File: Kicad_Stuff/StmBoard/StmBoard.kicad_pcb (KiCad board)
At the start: 4 copper layers, 103.6 x 50.6 mm, 46 parts, among them J1 USB_B_Mini, SW1 SW_DIP_x01, SW2 SW_DIP_x01, SW3 SW_DIP_x01, SW4 SW_DIP_x01, SW5 SW_DIP_x01, SW6 SW_DIP_x01, SW7 SW_DIP_x01, SW8 SW_DIP_x01, SW9 SW_DIP_x01, U1 STM32G031K8Tx, U13 MCP2221AxST, U2 LIS3DH, U8 MIC5504-3.3YM5, U9 L78L05_SO8, Y1 32Khz LSE

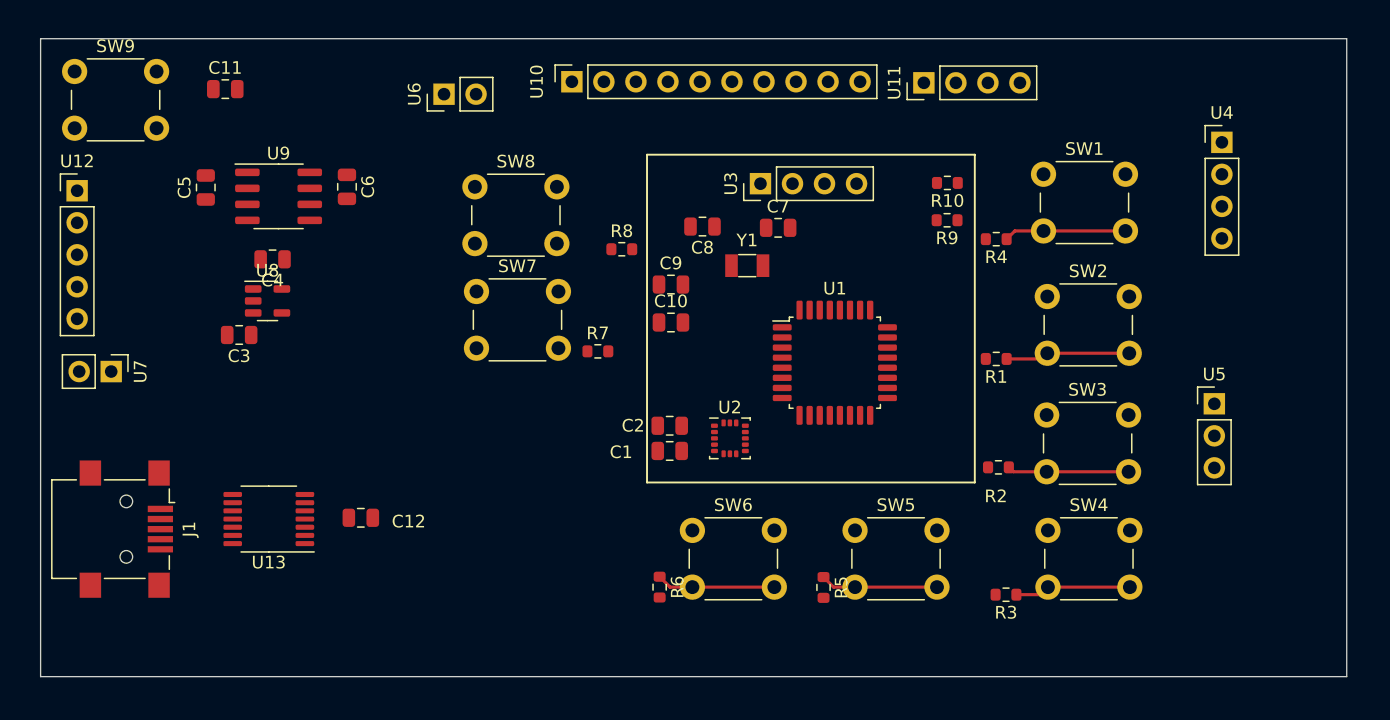
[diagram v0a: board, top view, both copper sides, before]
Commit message: quick commit
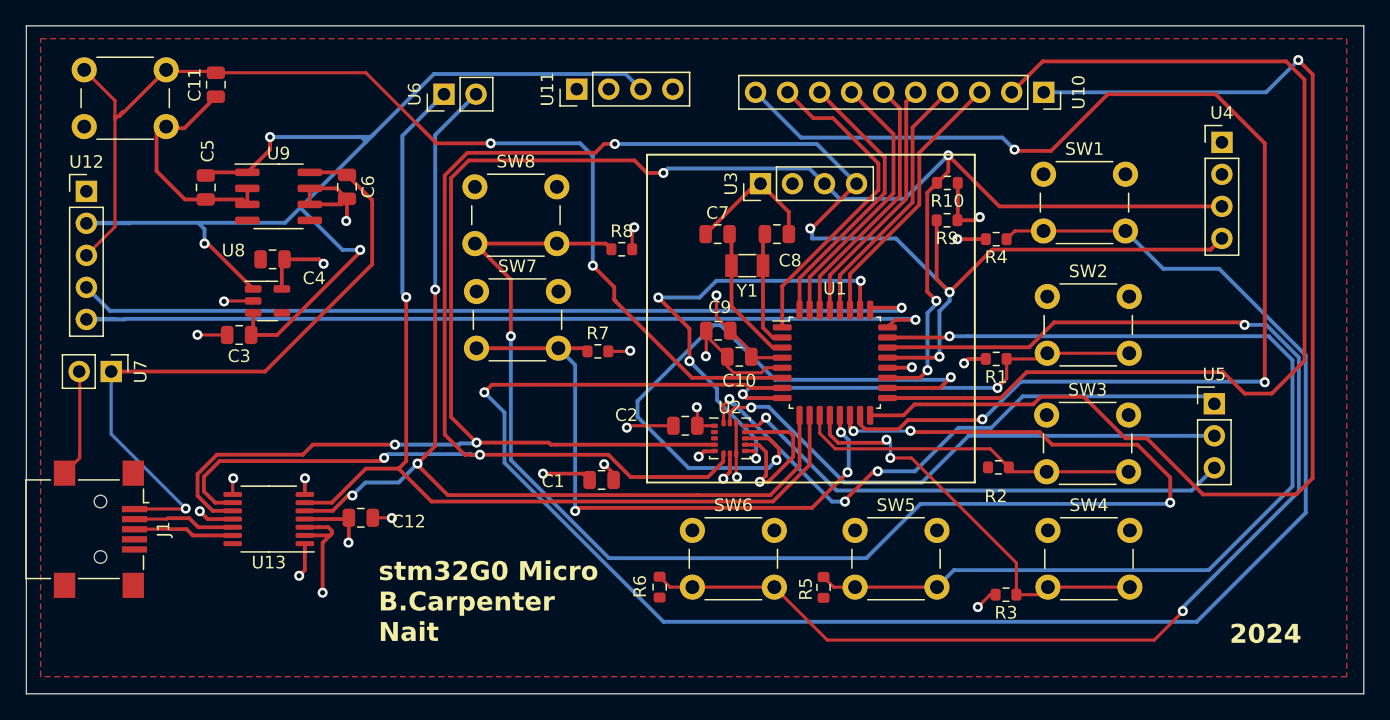
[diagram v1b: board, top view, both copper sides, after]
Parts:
- moved U10 37.4 mm to (154.3, 80.3), turned to -90 degrees
- moved U11 27.5 mm to (117.2, 80.1)
- moved C10 6.06 mm to (130.1, 101.3)
- moved C8 5.93 mm to (133.1, 91.6)
- moved C1 5.87 mm to (119.2, 111.1)
- moved C9 5.24 mm to (128.4, 99.3)
- moved C7 4.83 mm to (128.4, 91.6)
- moved J1 2.05 mm to (79.5, 115.0)
- moved C2 1.24 mm to (125.8, 106.8)
- moved C11 0.83 mm to (88.6, 79.8), turned to 90 degrees
- moved SW9 0.77 mm to (78.2, 78.6)
- moved U12 0.74 mm to (78.3, 88.2)
- turned C5 to -90 degrees
- turned Y1 to 180 degrees
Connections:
- J1 pad 4: unconnected-(J1-ID-Pad4) -> GND
- U13 pad 10: SWCLK -> /SCL
- U13 pad 9: SWDIO -> /SDA
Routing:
- net /SDA: track 0.00 -> 164.4 mm, vias 0 -> 6
- net /SCL: track 0.00 -> 157.1 mm, vias 0 -> 6
- net /A0: track 9.69 -> 143.1 mm, vias 0 -> 1
- net /A7: track 0.00 -> 116.7 mm, vias 0 -> 4
- net GND: track 0.00 -> 112.7 mm, vias 0 -> 19
- net Net-(U1-PB0): track 0.00 -> 99.3 mm, vias 0 -> 3
- net VCC: track 0.00 -> 96.5 mm, vias 0 -> 3
- net Net-(U1-PB1): track 0.00 -> 94.3 mm, vias 0 -> 1
- net /A5: track 9.44 -> 103.1 mm, vias 0 -> 2
- net /reset: track 0.00 -> 93.3 mm, vias 0 -> 2
- net Net-(U1-PB2): track 0.00 -> 82.8 mm
- net /RX_UASART2_VCOM: track 0.00 -> 78.8 mm, vias 0 -> 1
- net /TX_UASART2_VCOM: track 0.00 -> 78.1 mm, vias 0 -> 3
- net /A4: track 9.58 -> 84.0 mm, vias 0 -> 1
- net SWDIO: track 0.00 -> 71.3 mm, vias 0 -> 1
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- added copper zone on In2.Cu, net +3.3V
- added copper zone on F.Cu, net GND
- added copper zone on In1.Cu, net GND
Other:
- board size 103.6 x 50.6 mm -> 106.1 x 53 mm
- board text added: "2024"
- board text added: "stm32G0 Micro B.Carpenter Nait"
